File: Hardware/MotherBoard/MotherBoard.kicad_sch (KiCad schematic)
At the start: 24 parts, among them J1 POWER, J10 I/O_PWR, J13 USB_OTG, J2 I/O0, J5 I/O1, J6 EXTRN_CLCK, J9 Conn_02x02_Odd_Even, SW1 RESET_SW, SW2 ON_OFF, U1 AMS1117-5.0, X1 ACO-1MHz

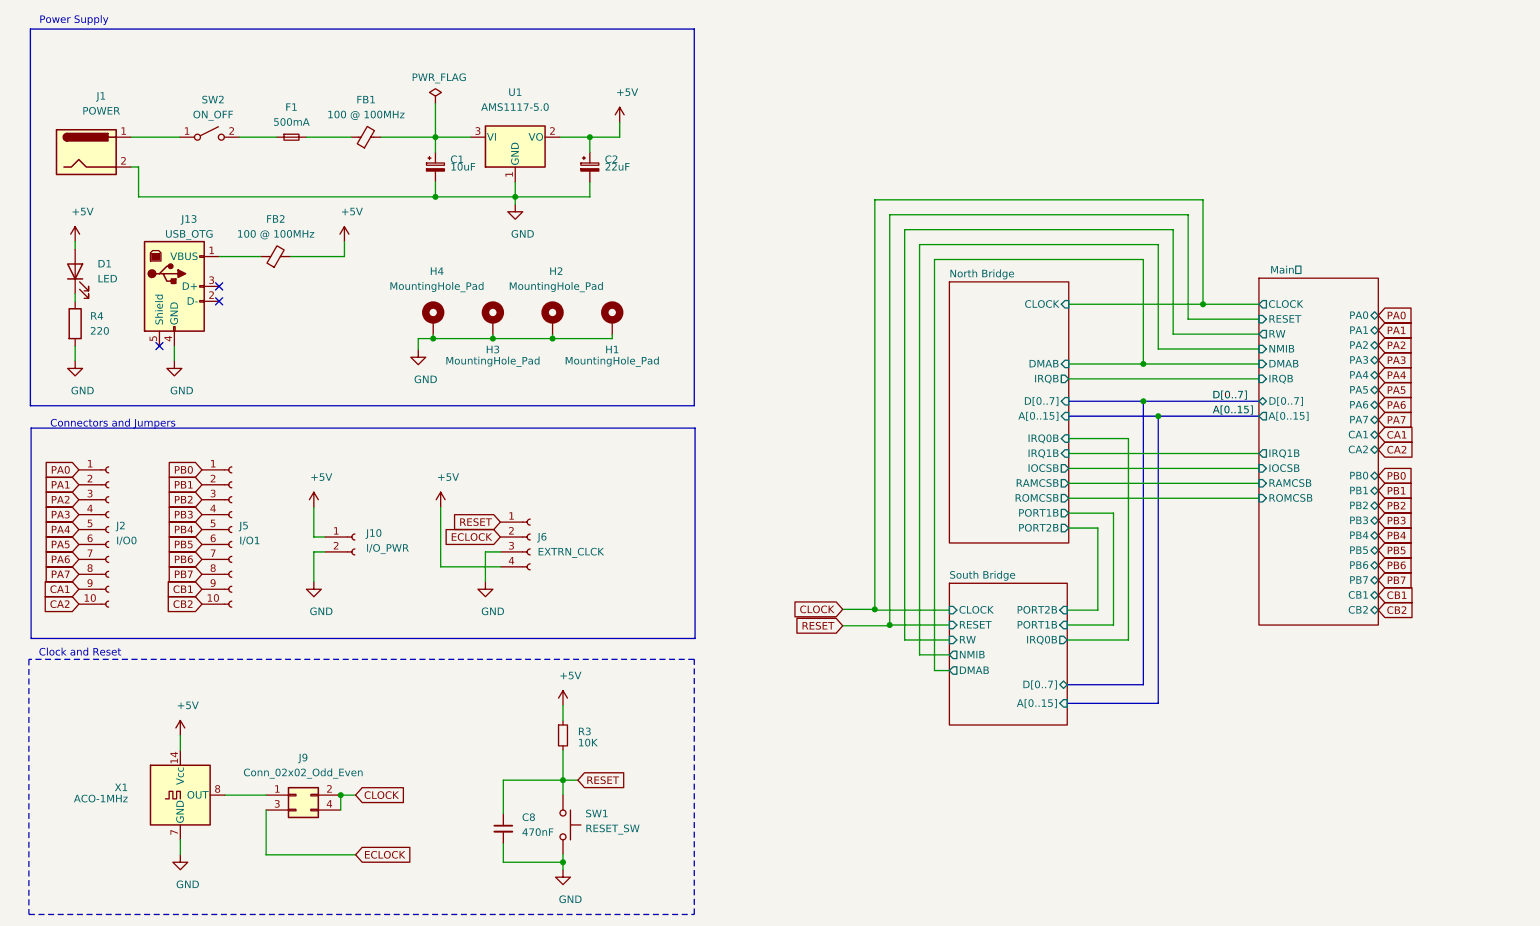
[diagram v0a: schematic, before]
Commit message: Fix
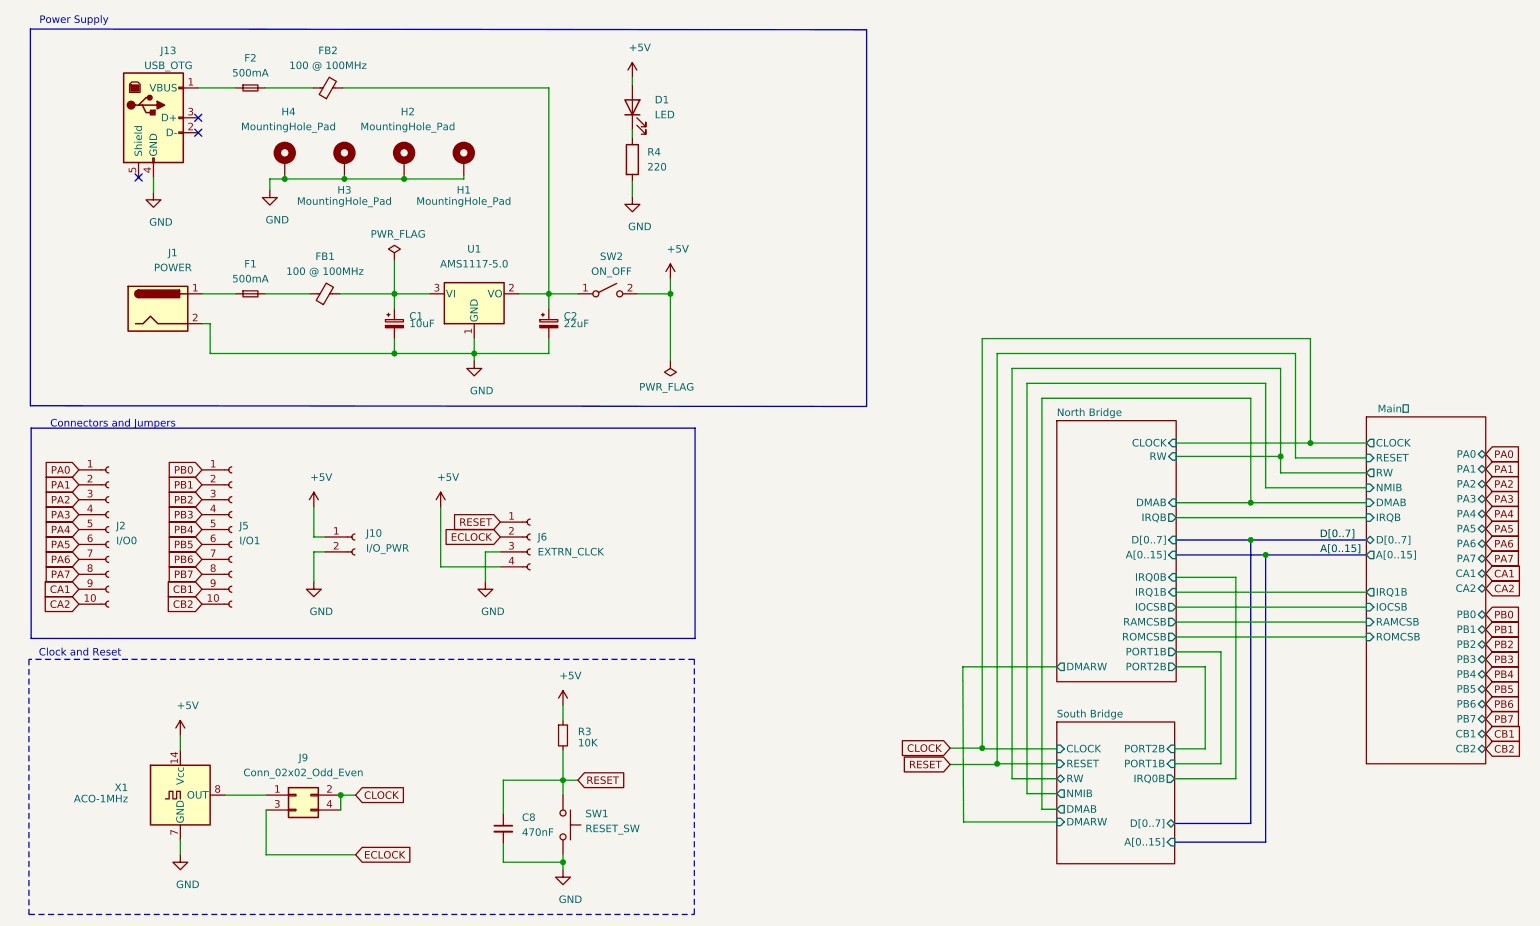
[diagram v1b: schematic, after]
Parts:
- added F2: 500mA, Resistor_THT:R_Box_L8.4mm_W2.5mm_P5.08mm, symbol Device:Fuse_Small
- U1: footprint Package_TO_SOT_SMD:SOT-223-3_TabPin2 -> Package_TO_SOT_THT:TO-220-3_Horizontal_TabDown
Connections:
- net +5V: now also SW2.2 (B); no longer C2.1, FB2.2, U1.2 (VO)
- net at J13.1 (VBUS): now also F2.1; no longer FB2.1
- net at SW2.1 (A): now also C2.1, FB2.2, U1.2 (VO); no longer J1.1
- net at F1.1: now also J1.1; no longer SW2.2 (B)
- new net: F2.2, FB2.1
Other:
- sheet North Bridge ports: added DMARW, RW; removed none
- sheet South Bridge ports: added DMARW; removed none
- title: Retro 6502 Mother Board -> Miniish
- moved on the sheet: C1, C2, D1, F1, FB1, FB2, H1, H2, H3, H4, J1, J13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
